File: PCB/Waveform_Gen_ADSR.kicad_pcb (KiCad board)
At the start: 2 copper layers, 50.8 x 22.9 mm, 28 parts, among them J6 WAVE_OUT, M1 Feather_M4_Express, U1 AD9833, U2 LMV116, U3 AD5245, X1 25.000MHZ

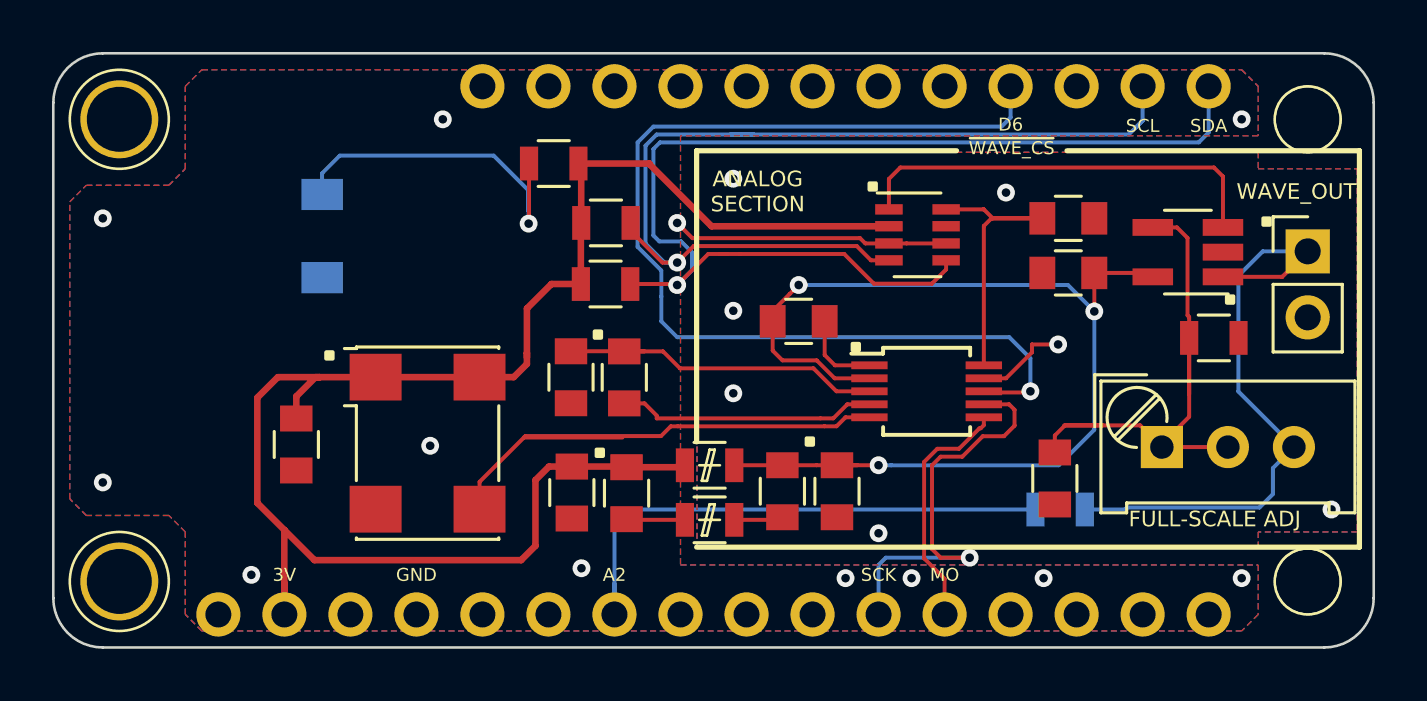
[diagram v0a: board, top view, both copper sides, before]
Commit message: update backup folder
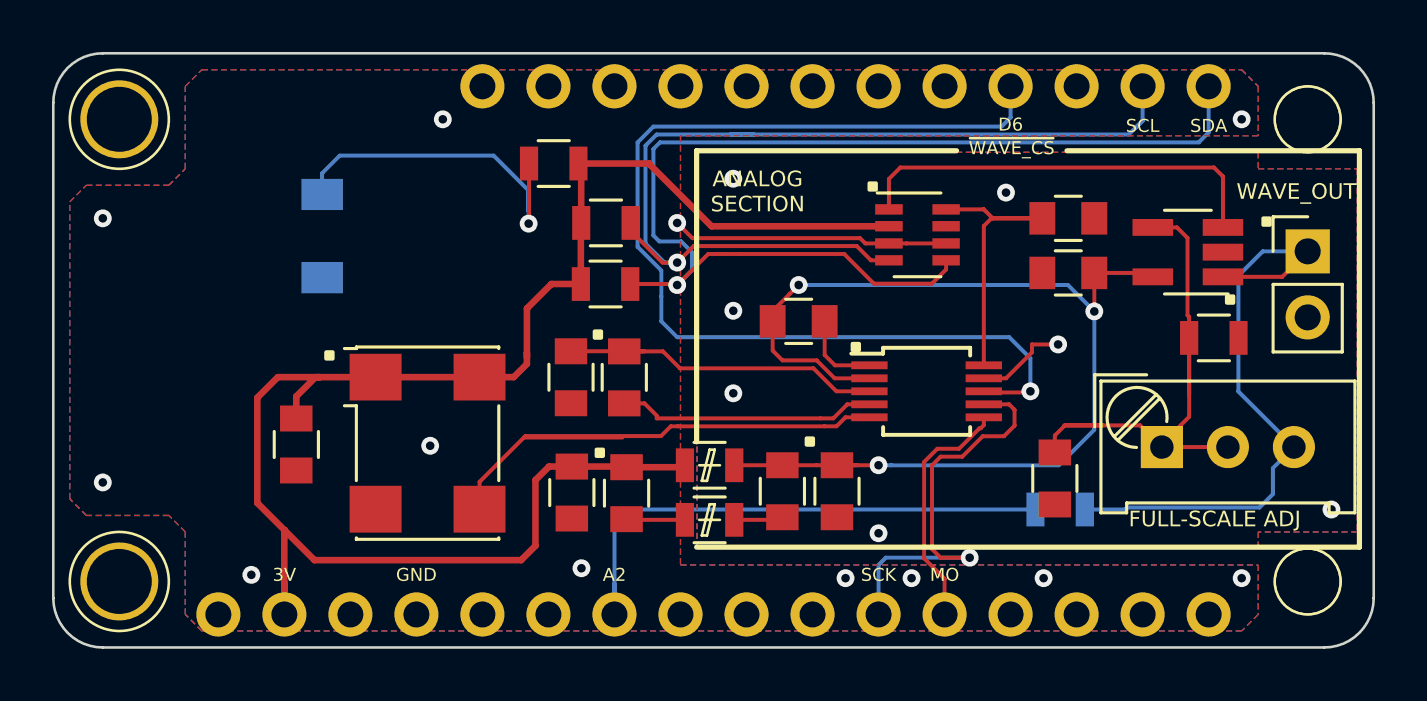
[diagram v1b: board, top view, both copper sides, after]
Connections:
- net /~WAVE_CS renamed /~{WAVE_CS}
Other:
- net class Default removed
- net class Power removed
- board text added: "AD9833 Precision Waveform Generator + 8-bit amplitude control (via I2C) + FeatherWing, 3.3v powered + 0.5Hz to 100kHz, 0.1Hz accuracy + Sine/Square/Triangle waveform + 3.3v buffered output + SPI interface for waveform gen (D6 = ~{CS})"
- board text added: "~{WAVE_CS}"
- board text removed: "AD9833 Precision Waveform Generator + 8-bit amplitude control (via I2C) + FeatherWing, 3.3v powered + 0.5Hz to 100kHz, 0.1Hz accuracy + Sine/Square/Triangle waveform + 3.3v buffered output + SPI interface for waveform gen (D6 = ~CS~)"
- board text removed: "~WAVE_CS"
